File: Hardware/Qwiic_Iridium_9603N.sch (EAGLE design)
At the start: 61 parts, among them J1 IRIDIUM_9603N, J10 STANDOFFS_M2X0.4_STEEL_6MM, J3 PTH, J6 ISP, J7 U.FL, J9 STANDOFFS_M2X0.4_STEEL_6MM, Q2 5.8A/30V/35mΩ, U1 ATTINY841SOIC, U2 LTC3225EDDB#TRMPBF, U3 ADM4210-1

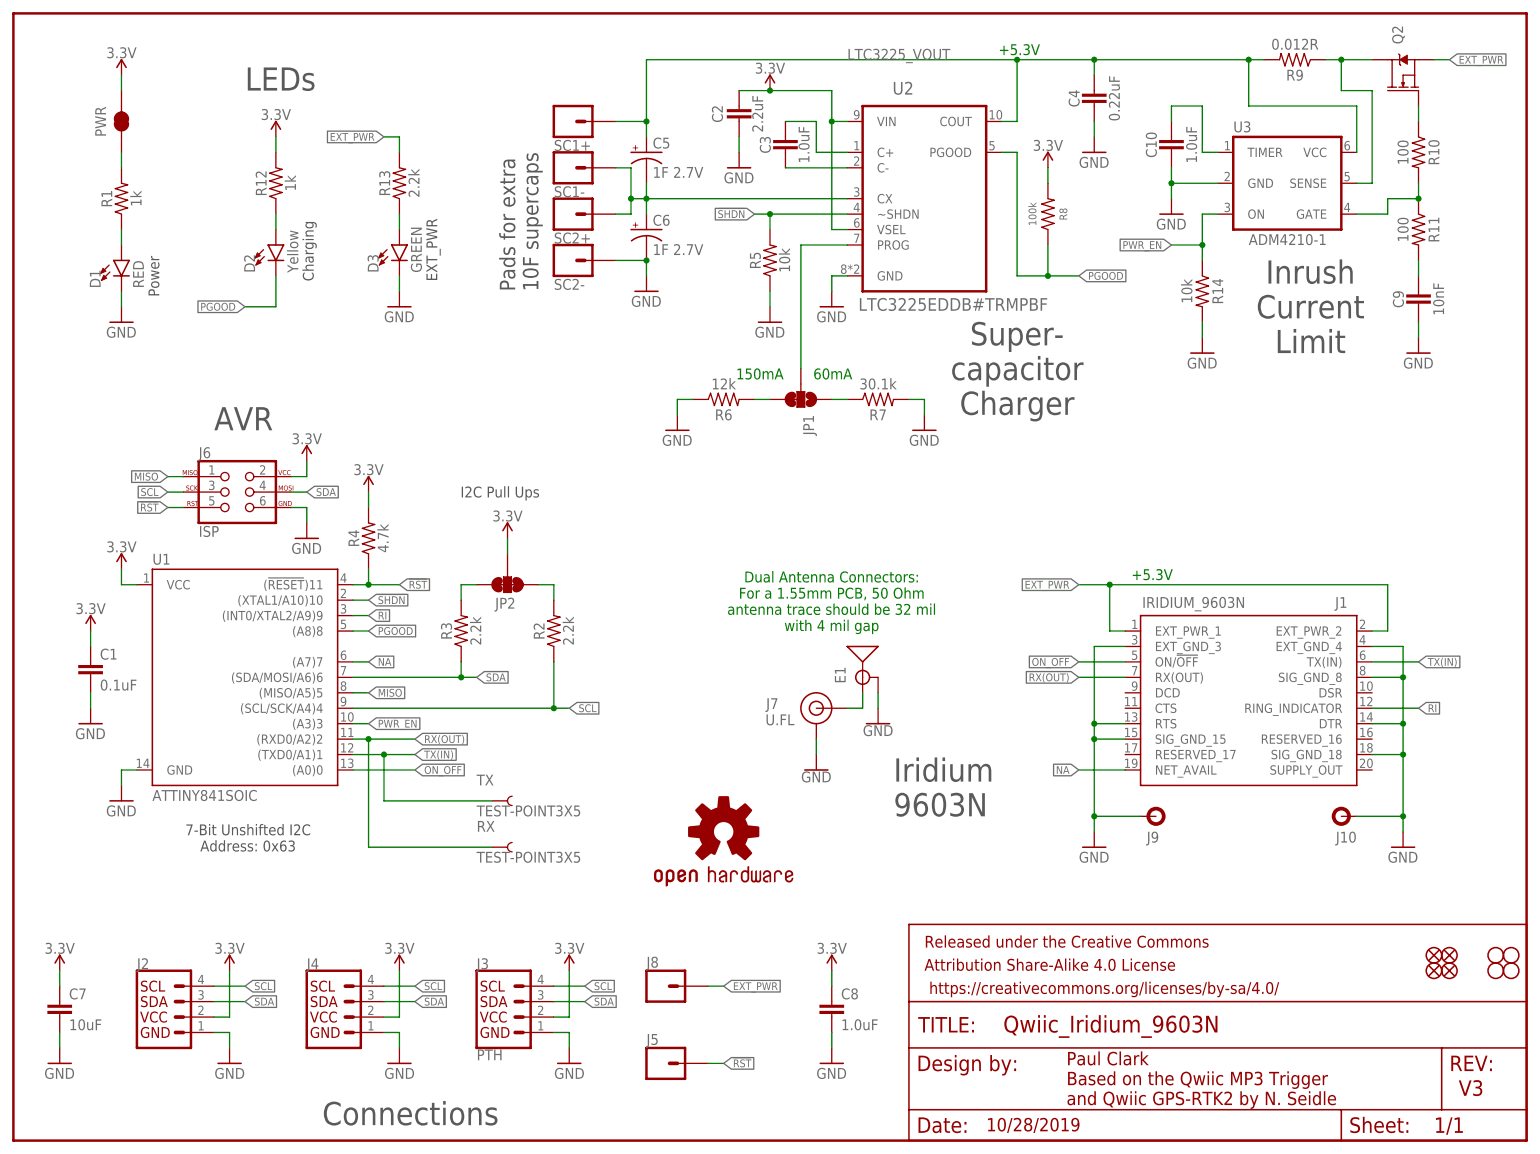
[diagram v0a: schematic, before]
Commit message: Adding x02 regular and production files.
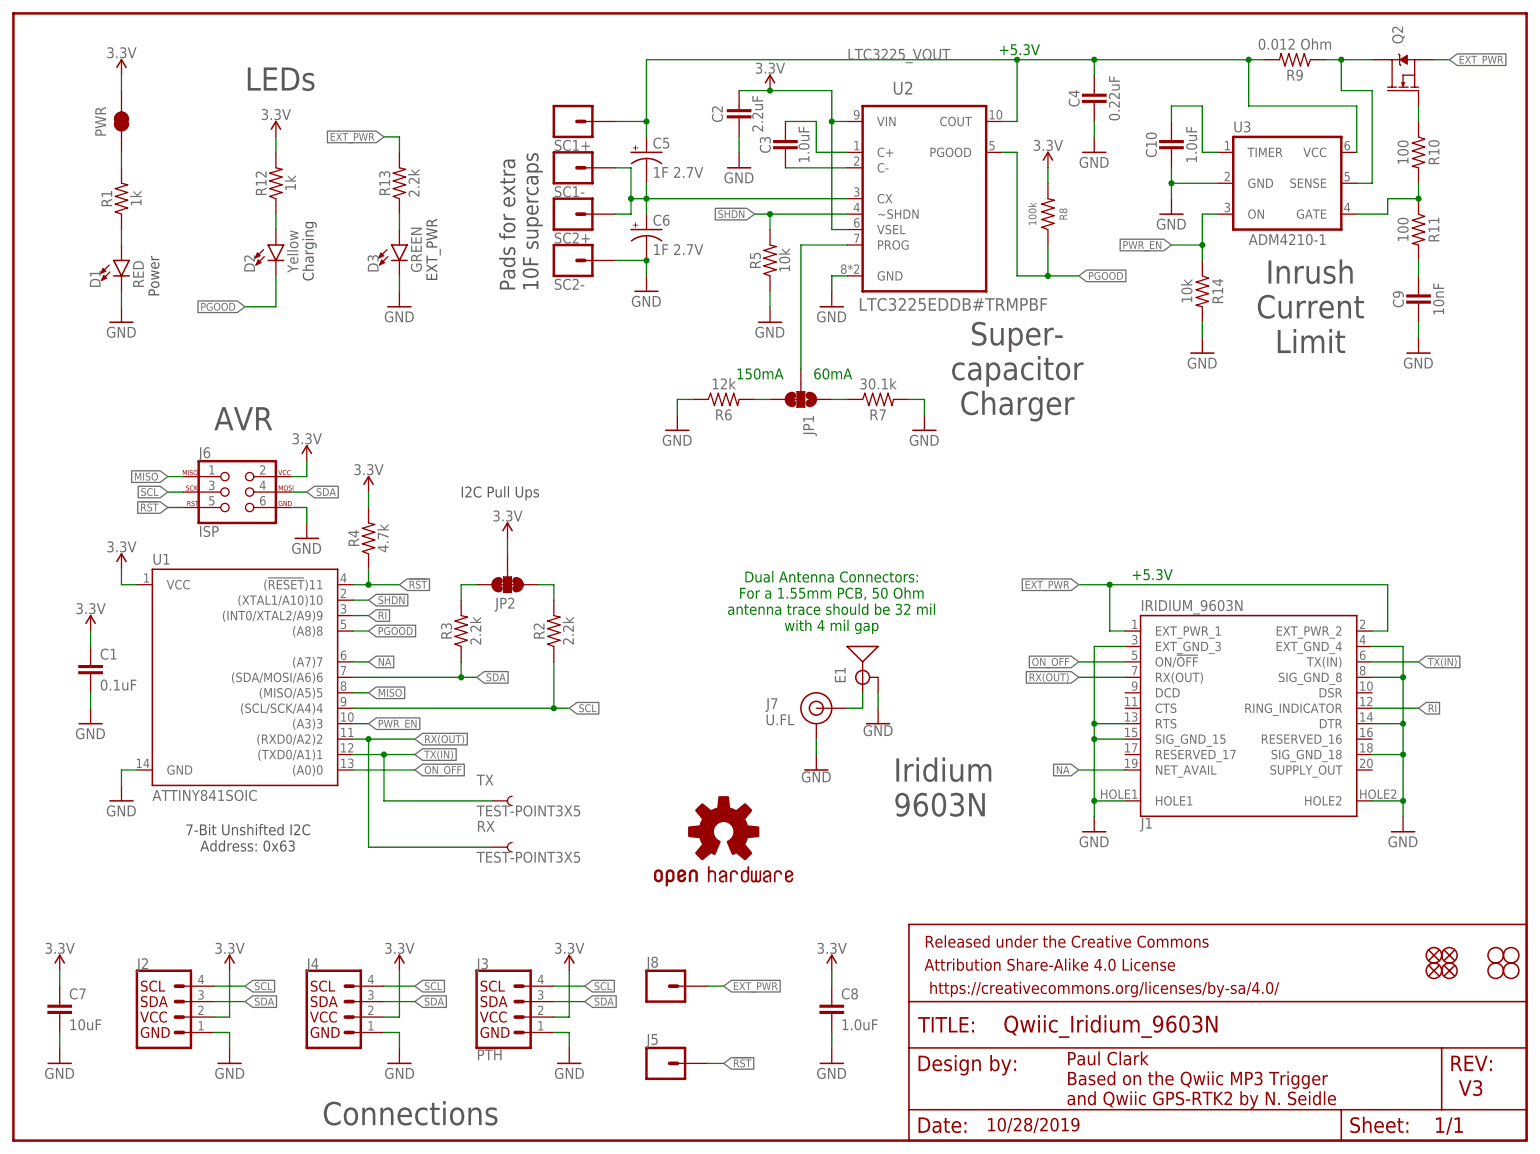
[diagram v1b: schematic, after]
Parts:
- removed J10, J9: STANDOFFS_M2X0.4_STEEL_6MM, New_Parts:STANDOFFS_M2X0.4_STEEL_6MM
- C5, C6: device New_Parts:1F-2.7V(PTH)CPOL-RADIAL-1H-2.7V -> SparkFun-Capacitors:1F-2.7V(PTH)CPOL-RADIAL-1H-2.7V
- J1: device New_Parts:IRIDIUM_9603N -> Qwiic_Iridium_9603N:IRIDIUM_9603N
- R1, R12: device SparkFun-Resistors:1KOHM-0603-1/10W-1% -> Qwiic_Iridium_9603N:1KOHM-0603-1/10W-1%
- R9: value 0.012R -> 0.012 Ohm; device New_Parts:RESISTOR_0603_12MILLIOHM0603 -> SparkFun-Resistors:RESISTOR0603
- U1: device New_Parts:ATTINY841SOIC -> Qwiic_Iridium_9603N:ATTINY841SOIC
- U2: device New_Parts:LTC3225EDDB-TRMPBFDFN300X200-10L -> Qwiic_Iridium_9603N:LTC3225EDDB-TRMPBFDFN300X200-10L
- U3: device New_Parts:ADM4210-1 -> Qwiic_Iridium_9603N:ADM4210-1
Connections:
- net GND: now also J1.HOLE1, J1.HOLE2; no longer J10.1, J9.1
